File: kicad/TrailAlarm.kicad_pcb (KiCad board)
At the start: 2 copper layers, 71.1 x 36.2 mm, 57 parts, among them IC1 MAX865EUA+T, J1 Conn_01x03, J2 Conn_01x01_Male, J3 Adafruit ADS1115, J4 Bat, Q1 2N3904, SW1 SW_DIP_x01, U1 TLC274, U2 TL074, U3 PocketBeagle, U5 AD620

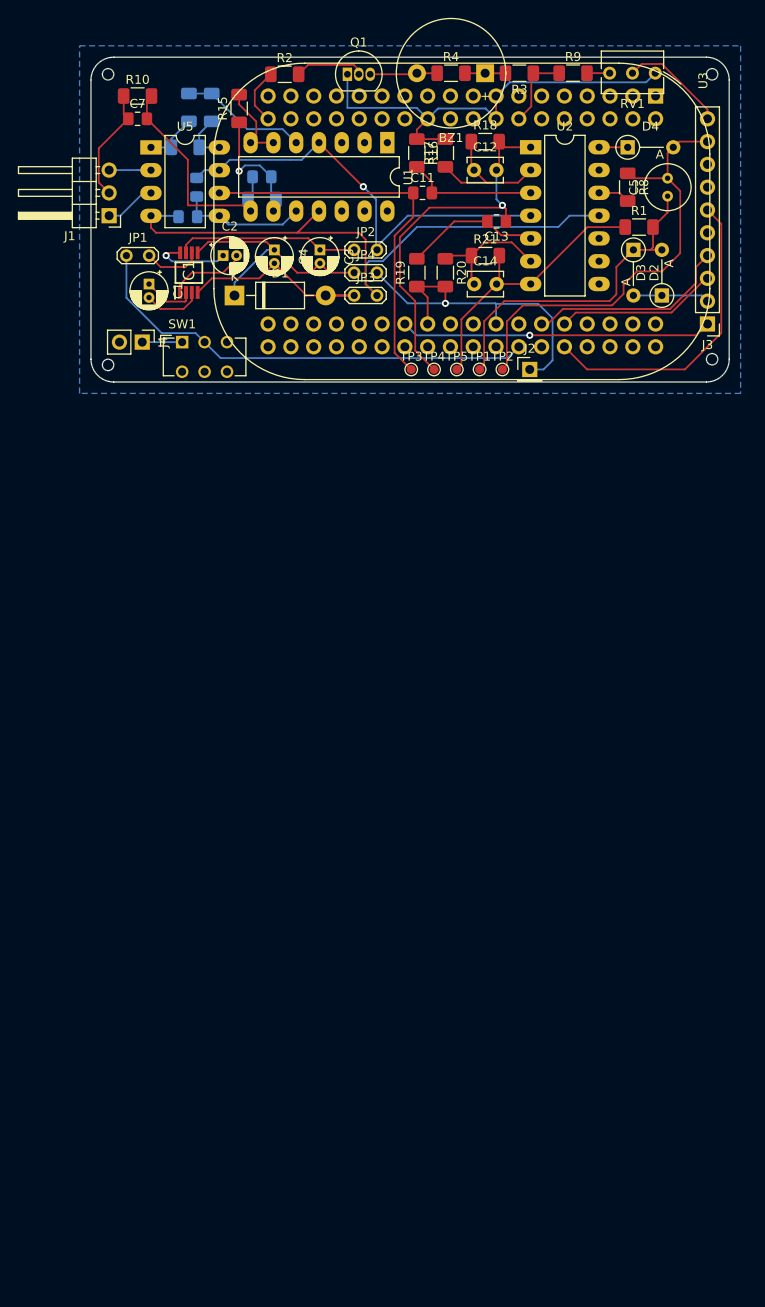
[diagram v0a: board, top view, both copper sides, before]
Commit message: Export gerber files
- Reflow
- print to pdf
- generate gerber/drill files for fab
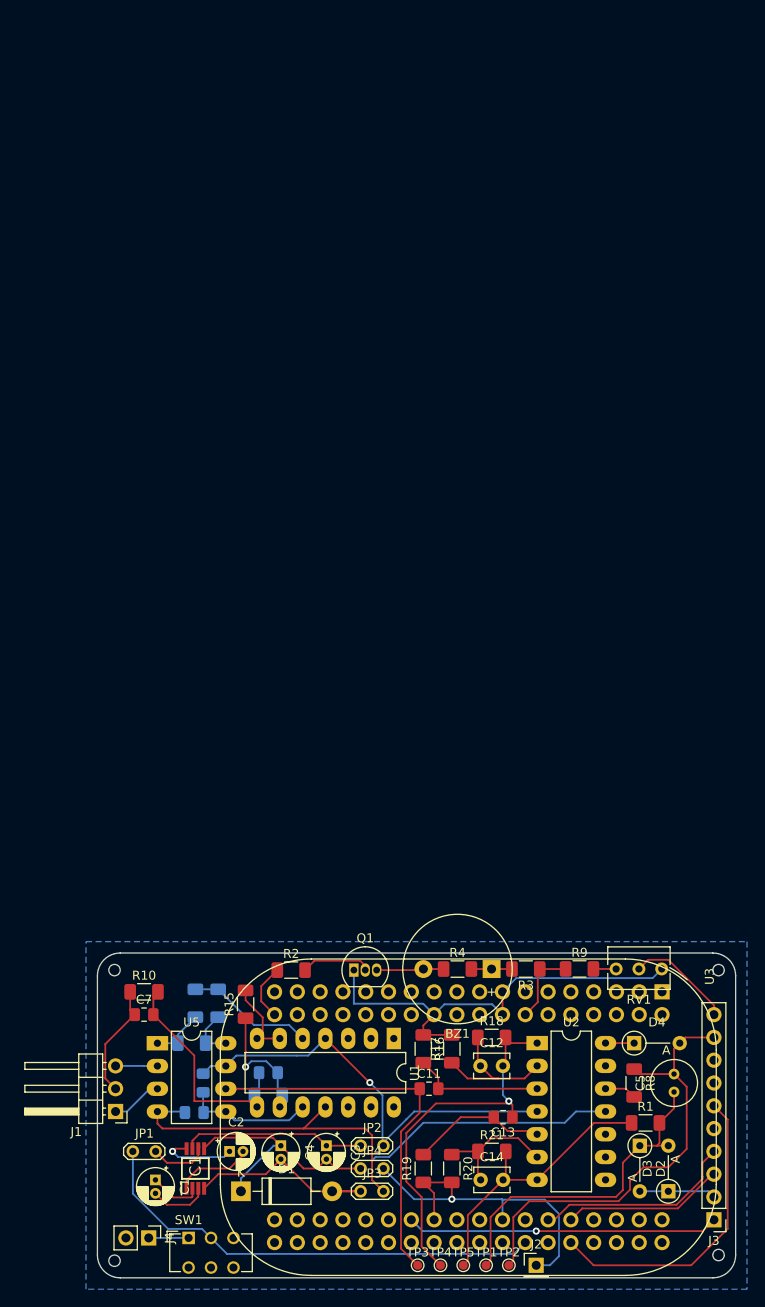
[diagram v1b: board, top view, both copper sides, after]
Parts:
- moved BZ1 99.8 mm to (160.8, 114.3)
- moved C1 99.8 mm to (123.4, 137.8)
- moved C11 99.8 mm to (153.9, 127.6)
- moved C12 99.8 mm to (159.6, 125.1)
- moved C14 99.8 mm to (159.6, 137.8)
- moved C3 99.8 mm to (142.4, 134.0)
- moved C4 99.8 mm to (137.4, 134.0)
- moved C7 99.8 mm to (122.1, 119.4)
- moved C8 99.8 mm to (136.0, 125.9)
- moved C9 99.8 mm to (128.7, 127.0)
- moved D1 99.8 mm to (132.9, 139.1)
- moved D2 99.8 mm to (177.4, 134.0)
- moved D3 99.8 mm to (180.5, 139.1)
- moved D4 99.8 mm to (176.7, 122.6)
- moved J1 99.8 mm to (118.9, 130.2)
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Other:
- outline, holes or cut-outs redrawn
